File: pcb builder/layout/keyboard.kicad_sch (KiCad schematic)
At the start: 154 parts

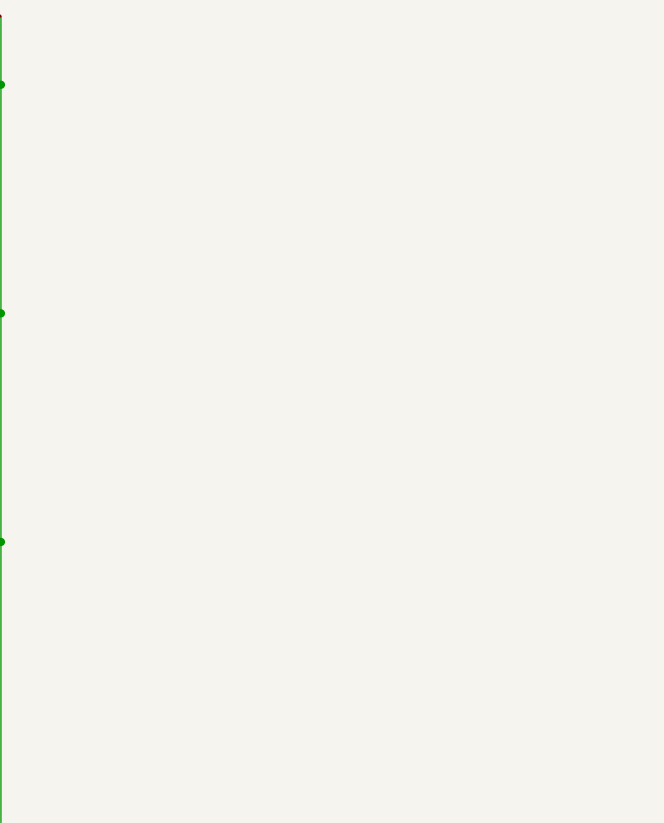
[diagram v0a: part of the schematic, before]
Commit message: submoduling all folders KEKW
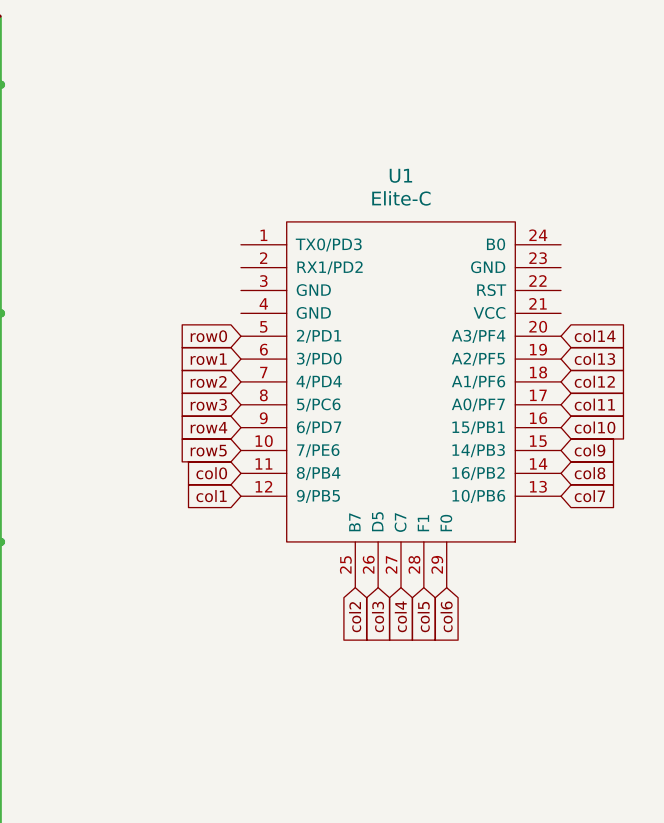
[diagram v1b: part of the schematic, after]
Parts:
- added U1: Elite-C, symbol keebio:Elite-C
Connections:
- net col0: now also U1.11 (8/PB4)
- net col1: now also U1.12 (9/PB5)
- net col10: now also U1.16 (15/PB1)
- net col11: now also U1.17 (A0/PF7)
- net col12: now also U1.18 (A1/PF6)
- net col13: now also U1.19 (A2/PF5)
- net col14: now also U1.20 (A3/PF4)
- net col2: now also U1.25 (B7)
- net col3: now also U1.26 (D5)
- net col4: now also U1.27 (C7)
- net col5: now also U1.28 (F1)
- net col6: now also U1.29 (F0)
- net col7: now also U1.13 (10/PB6)
- net col8: now also U1.14 (16/PB2)
- net col9: now also U1.15 (14/PB3)
- net row0: now also U1.5 (2/PD1)
- net row1: now also U1.6 (3/PD0)
- net row2: now also U1.7 (4/PD4)
- net row3: now also U1.8 (5/PC6)
- net row4: now also U1.9 (6/PD7)
- net row5: now also U1.10 (7/PE6)
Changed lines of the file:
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@@
+    )
+  )
+  (global_label "row1" (shape input) (at 427.99 54.61 180)
+    (effects (font (size 1.27 1.27)) (justify right))
+    (property "Intersheetrefs" "${INTERSHEET_REFS}" (at 427.99 54.61 0)
+      (effects (font (size 1.27 1.27)) hide)
+    )
+  )
+  (global_label "col4" (shape input) (at 445.77 80.01 270)
+    (effects (font (size 1.27 1.27)) (justify right))
+    (property "Intersheetrefs" "${INTERSHEET_REFS}" (at 445.77 80.01 0)
+      (effects (font (size 1.27 1.27)) hide)
+    )
+  )
+  (global_label "col8" (shape input) (at 463.55 67.31 0)
+    (effects (font (size 1.27 1.27)) (justify left))
+    (property "Intersheetrefs" "${INTERSHEET_REFS}" (at 463.55 67.31 0)
+      (effects (font (size 1.27 1.27)) hide)
     )
   )
@@
     )
   )
+  (global_label "row0" (shape input) (at 427.99 52.07 180)
+    (effects (font (size 1.27 1.27)) (justify right))
+    (property "Intersheetrefs" "${INTERSHEET_REFS}" (at 427.99 52.07 0)
+      (effects (font (size 1.27 1.27)) hide)
+    )
+  )
   (global_label "col13" (shape input) (at 375.92 16.51 180)
     (effects (font (size 1.27 1.27)) (justify right))
@@
     )
   )
+  (global_label "row5" (shape input) (at 427.99 64.77 180)
+    (effects (font (size 1.27 1.27)) (justify right))
+    (property "Intersheetrefs" "${INTERSHEET_REFS}" (at 427.99 64.77 0)
+      (effects (font (size 1.27 1.27)) hide)
+    )
+  )
   (global_label "col6" (shape input) (at 198.12 16.51 180)
     (effects (font (size 1.27 1.27)) (justify right))
@@
     )
   )
+  (global_label "row3" (shape input) (at 427.99 59.69 180)
+    (effects (font (size 1.27 1.27)) (justify right))
+    (property "Intersheetrefs" "${INTERSHEET_REFS}" (at 427.99 59.69 0)
+      (effects (font (size 1.27 1.27)) hide)
+    )
+  )
+  (global_label "col14" (shape input) (at 463.55 52.07 0)
+    (effects (font (size 1.27 1.27)) (justify left))
+    (property "Intersheetrefs" "${INTERSHEET_REFS}" (at 463.55 52.07 0)
+      (effects (font (size 1.27 1.27)) hide)
+    )
+  )
   (global_label "row1" (shape input) (at 22.86 60.96 180)
     (effects (font (size 1.27 1.27)) (justify right))
@@
     )
   )
+  (global_label "col2" (shape input) (at 440.69 80.01 270)
+    (effects (font (size 1.27 1.27)) (justify right))
+    (property "Intersheetrefs" "${INTERSHEET_REFS}" (at 440.69 80.01 0)
+      (effects (font (size 1.27 1.27)) hide)
+    )
+  )
+  (global_label "col5" (shape input) (at 448.31 80.01 270)
+    (effects (font (size 1.27 1.27)) (justify right))
+    (property "Intersheetrefs" "${INTERSHEET_REFS}" (at 448.31 80.01 0)
+      (effects (font (size 1.27 1.27)) hide)
+    )
+  )
   (global_label "col5" (shape input) (at 172.72 16.51 180)
     (effects (font (size 1.27 1.27)) (justify right))
@@
     )
   )
+  (global_label "col10" (shape input) (at 463.55 62.23 0)
+    (effects (font (size 1.27 1.27)) (justify left))
+    (property "Intersheetrefs" "${INTERSHEET_REFS}" (at 463.55 62.23 0)
+      (effects (font (size 1.27 1.27)) hide)
+    )
+  )
+  (global_label "col13" (shape input) (at 463.55 54.61 0)
+    (effects (font (size 1.27 1.27)) (justify left))
+    (property "Intersheetrefs" "${INTERSHEET_REFS}" (at 463.55 54.61 0)
+      (effects (font (size 1.27 1.27)) hide)
+    )
+  )
+  (global_label "col7" (shape input) (at 463.55 69.85 0)
+    (effects (font (size 1.27 1.27)) (justify left))
+    (property "Intersheetrefs" "${INTERSHEET_REFS}" (at 463.55 69.85 0)
+      (effects (font (size 1.27 1.27)) hide)
+    )
+  )
+  (global_label "col11" (shape input) (at 463.55 59.69 0)
+    (effects (font (size 1.27 1.27)) (justify left))
+    (property "Intersheetrefs" "${INTERSHEET_REFS}" (at 463.55 59.69 0)
+      (effects (font (size 1.27 1.27)) hide)
+    )
+  )
+  (global_label "col0" (shape input) (at 427.99 67.31 180)
+    (effects (font (size 1.27 1.27)) (justify right))
+    (property "Intersheetrefs" "${INTERSHEET_REFS}" (at 427.99 67.31 0)
+      (effects (font (size 1.27 1.27)) hide)
+    )
+  )
+  (global_label "row2" (shape input) (at 427.99 57.15 180)
+    (effects (font (size 1.27 1.27)) (justify right))
+    (property "Intersheetrefs" "${INTERSHEET_REFS}" (at 427.99 57.15 0)
+      (effects (font (size 1.27 1.27)) hide)
+    )
+  )
   (global_label "col14" (shape input) (at 401.32 16.51 180)
     (effects (font (size 1.27 1.27)) (justify right))
@@
     )
   )
+  (global_label "row4" (shape input) (at 427.99 62.23 180)
+    (effects (font (size 1.27 1.27)) (justify right))
+    (property "Intersheetrefs" "${INTERSHEET_REFS}" (at 427.99 62.23 0)
+      (effects (font (size 1.27 1.27)) hide)
+    )
+  )
   (global_label "row5" (shape input) (at 22.86 162.56 180)
     (effects (font (size 1.27 1.27)) (justify right))
@@
     )
   )
+  (global_label "col9" (shape input) (at 463.55 64.77 0)
+    (effects (font (size 1.27 1.27)) (justify left))
+    (property "Intersheetrefs" "${INTERSHEET_REFS}" (at 463.55 64.77 0)
+      (effects (font (size 1.27 1.27)) hide)
+    )
+  )
   (global_label "col7" (shape input) (at 223.52 16.51 180)
     (effects (font (size 1.27 1.27)) (justify right))
@@
     )
   )
+  (global_label "col3" (shape input) (at 443.23 80.01 270)
+    (effects (font (size 1.27 1.27)) (justify right))
+    (property "Intersheetrefs" "${INTERSHEET_REFS}" (at 443.23 80.01 0)
+      (effects (font (size 1.27 1.27)) hide)
+    )
+  )
+  (global_label "col12" (shape input) (at 463.55 57.15 0)
+    (effects (font (size 1.27 1.27)) (justify left))
+    (property "Intersheetrefs" "${INTERSHEET_REFS}" (at 463.55 57.15 0)
+      (effects (font (size 1.27 1.27)) hide)
+    )
+  )
+  (global_label "col6" (shape input) (at 450.85 80.01 270)
+    (effects (font (size 1.27 1.27)) (justify right))
+    (property "Intersheetrefs" "${INTERSHEET_REFS}" (at 450.85 80.01 0)
+      (effects (font (size 1.27 1.27)) hide)
+    )
+  )
+  (global_label "col1" (shape input) (at 427.99 69.85 180)
+    (effects (font (size 1.27 1.27)) (justify right))
+    (property "Intersheetrefs" "${INTERSHEET_REFS}" (at 427.99 69.85 0)
+      (effects (font (size 1.27 1.27)) hide)
+    )
+  )
   (symbol (lib_id "Device:D_Small") (at 135.89 83.82 90) (unit 1)
     (in_bom yes) (on_board yes) (dnp no)
@@
         )
       )
+    )
+  )
+  (symbol (lib_id "keebio:Elite-C") (at 445.77 55.88 0) (unit 1)
+    (in_bom yes) (on_board yes) (dnp no) (fields_autoplaced)
+    (property "Reference" "U1" (at 445.77 34.29 0)
+      (effects (font (size 1.524 1.524)))
+    )
+    (property "Value" "Elite-C" (at 445.77 36.83 0)
+      (effects (font (size 1.524 1.524)))
+    )
+    (property "Footprint" "" (at 472.44 119.38 90)
+      (effects (font (size 1.524 1.524)) hide)
+    )
+    (property "Datasheet" "" (at 472.44 119.38 90)
+      (effects (font (size 1.524 1.524)) hide)
+    )
+    (pin "1")
+    (pin "10")
+    (pin "11")
+    (pin "12")
+    (pin "13")
+    (pin "14")
+    (pin "15")
+    (pin "16")
+    (pin "17")
+    (pin "18")
+    (pin "19")
+    (pin "2")
+    (pin "20")
+    (pin "21")
+    (pin "22")
+    (pin "23")
+    (pin "24")
+    (pin "25")
+    (pin "26")
+    (pin "27")
+    (pin "28")
+    (pin "29")
+    (pin "3")
+    (pin "4")
+    (pin "5")
+    (pin "6")
+    (pin "7")
+    (pin "8")
+    (pin "9")
+    (instances
+      (project "keyboard"
+        (path "/218ad51d-6f09-4269-b673-c44cb9c7d5b4"
+          (reference "U1") (unit 1)
+        )
+      )
